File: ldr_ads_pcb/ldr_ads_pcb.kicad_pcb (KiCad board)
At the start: 2 copper layers, 4 parts

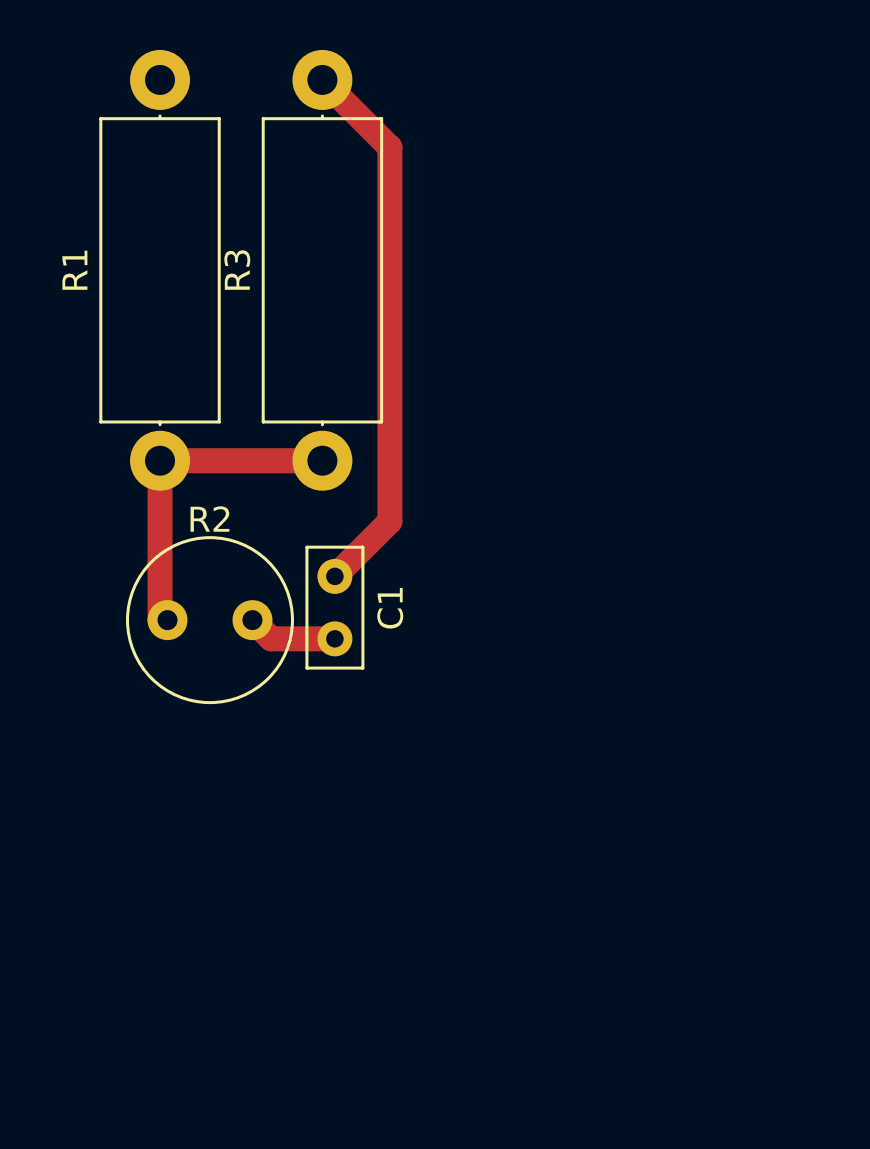
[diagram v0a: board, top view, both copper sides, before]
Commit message: feat: ready pcb
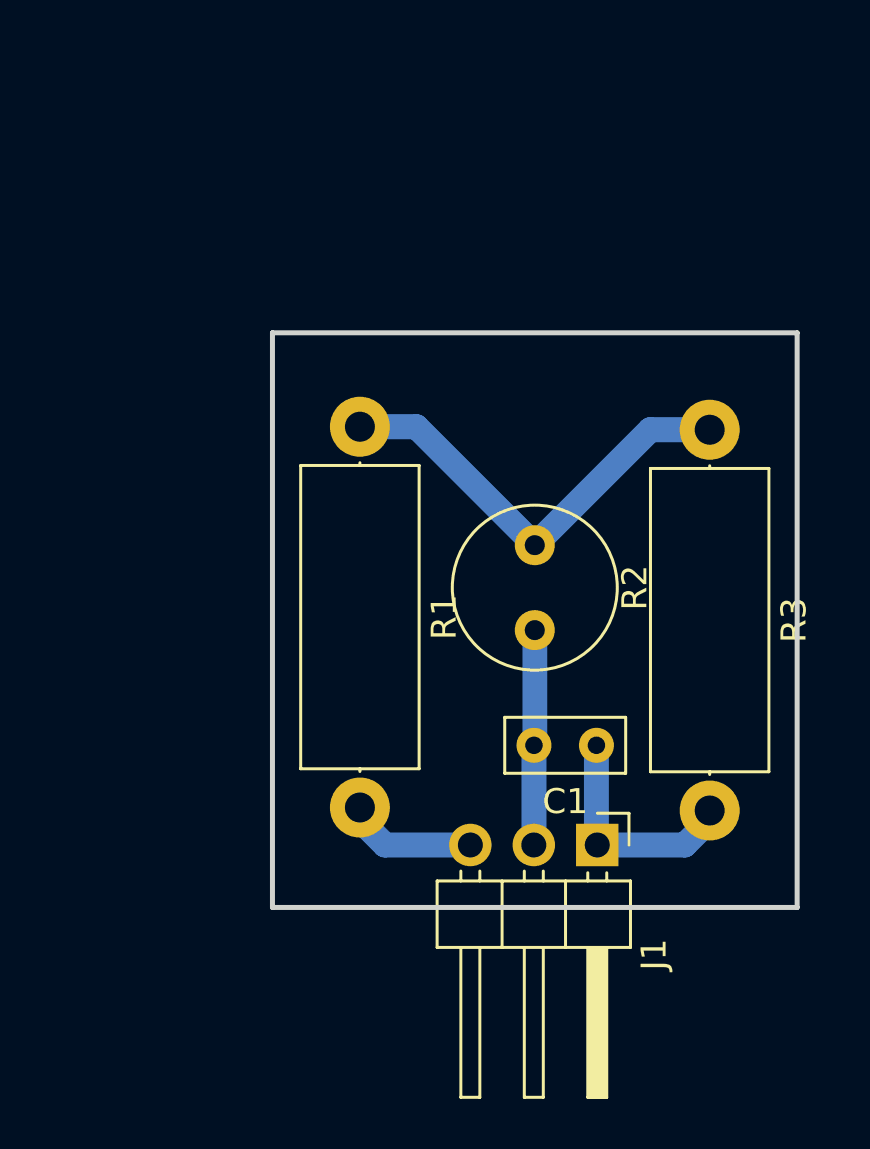
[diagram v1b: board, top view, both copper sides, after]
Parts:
- added J1: Conn_01x03, Connector_PinHeader_2.54mm:PinHeader_1x03_P2.54mm_Horizontal, F.Cu at (48.5, 45.0)
- moved R3 15.5 mm to (53.0, 28.4), turned to -90 degrees
- moved R2 15.0 mm to (46.0, 33.0), turned to -90 degrees
- moved C1 12.5 mm to (48.5, 41.0), turned to 180 degrees
- moved R1 8.11 mm to (39.0, 28.3), turned to -90 degrees
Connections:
- net Net-(C1-Pad1) renamed /out
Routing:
- net /out: track 21.9 -> 9.34 mm
- net +3.3V: track 0.00 -> 5.33 mm
- net GND: track 3.61 -> 8.63 mm
- net Net-(R1-Pad1): track 13.1 -> 18.0 mm
- added copper zone on B.Cu, net GND
- added copper zone on F.Cu, net GND
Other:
- board outline added: 21 x 23 mm
